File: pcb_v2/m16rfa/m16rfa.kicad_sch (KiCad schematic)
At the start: 58 parts, among them J1 S16A, J10 bus_rf16_3, J2 S16A, J3 SR8A, J5 S16A, J6 S16A, J7 S16A, J8 bus_rf16_1, J9 bus_rf16_2, U1 74LS125, U10 74LS244, U11 74LS244, U13 74LS02, U14 74LS04, U2 74LS193, U21 74LS08, U22 74LS138, U23 74LS138, U24 74LS32, U25 74LS00, U26 74LS138, U27 74LS138, U28 74LS138, U29 74LS138, U3 74LS138, U4 74LS08, U5 74LS04, U6 74LS08, U7 74LS244, U8 74LS244, U9 74LS244

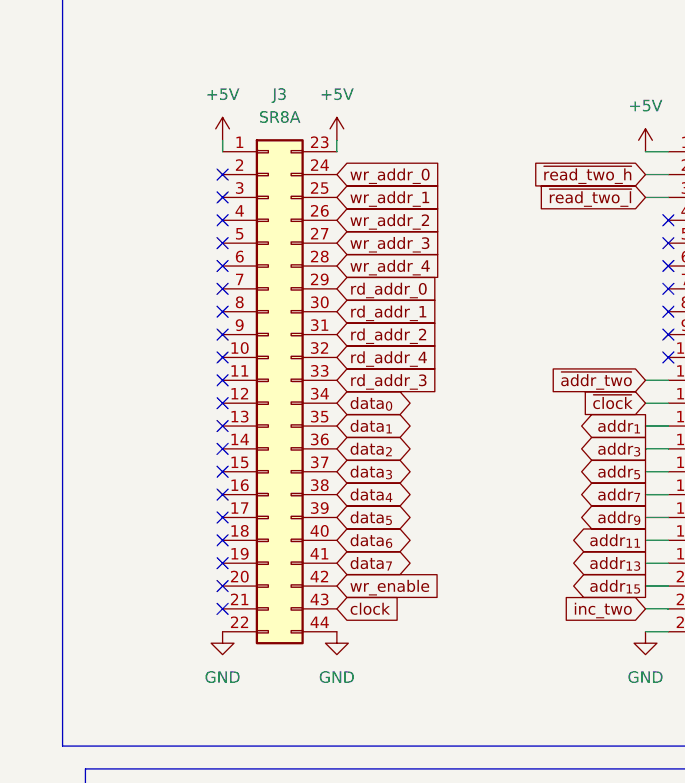
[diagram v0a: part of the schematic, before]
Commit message: .
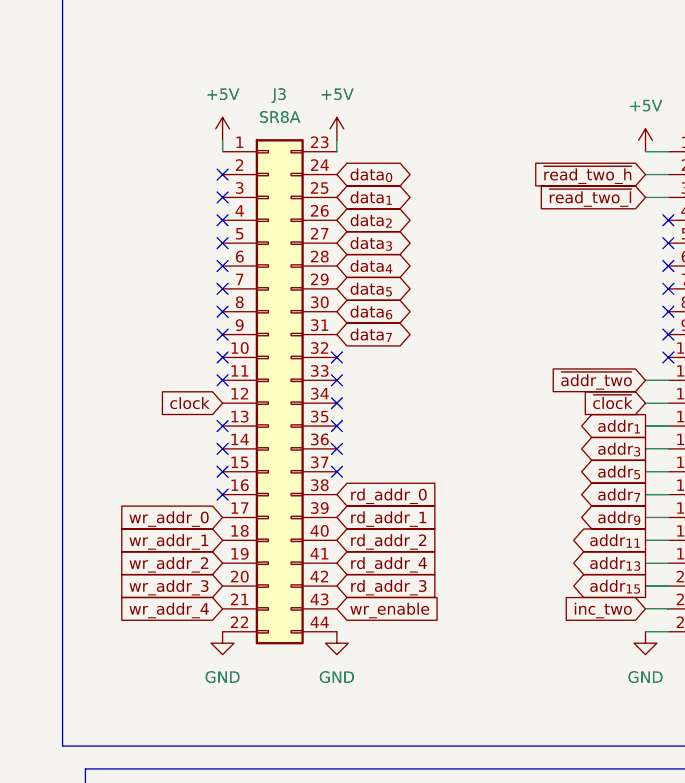
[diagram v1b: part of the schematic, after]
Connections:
- net clock: now also J3.12 (Pin_12); no longer J3.43 (Pin_43)
- net data_{0}: now also J3.24 (Pin_24); no longer J3.34 (Pin_34)
- net data_{1}: now also J3.25 (Pin_25); no longer J3.35 (Pin_35)
- net data_{2}: now also J3.26 (Pin_26); no longer J3.36 (Pin_36)
- net data_{3}: now also J3.27 (Pin_27); no longer J3.37 (Pin_37)
- net data_{4}: now also J3.28 (Pin_28); no longer J3.38 (Pin_38)
- net data_{5}: now also J3.29 (Pin_29); no longer J3.39 (Pin_39)
- net data_{6}: now also J3.30 (Pin_30); no longer J3.40 (Pin_40)
- net data_{7}: now also J3.31 (Pin_31); no longer J3.41 (Pin_41)
- net rd_addr_0: now also J3.38 (Pin_38); no longer J3.29 (Pin_29)
- net rd_addr_1: now also J3.39 (Pin_39); no longer J3.30 (Pin_30)
- net rd_addr_2: now also J3.40 (Pin_40); no longer J3.31 (Pin_31)
- net rd_addr_3: now also J3.42 (Pin_42); no longer J3.33 (Pin_33)
- net rd_addr_4: now also J3.41 (Pin_41); no longer J3.32 (Pin_32)
- net wr_addr_0: now also J3.17 (Pin_17); no longer J3.24 (Pin_24)
- net wr_addr_1: now also J3.18 (Pin_18); no longer J3.25 (Pin_25)
- net wr_addr_2: now also J3.19 (Pin_19); no longer J3.26 (Pin_26)
- net wr_addr_3: now also J3.20 (Pin_20); no longer J3.27 (Pin_27)
- net wr_addr_4: now also J3.21 (Pin_21); no longer J3.28 (Pin_28)
- net wr_enable: now also J3.43 (Pin_43); no longer J3.42 (Pin_42)
